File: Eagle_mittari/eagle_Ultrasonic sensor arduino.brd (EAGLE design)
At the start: 69.5 x 55.9 mm, 3 parts

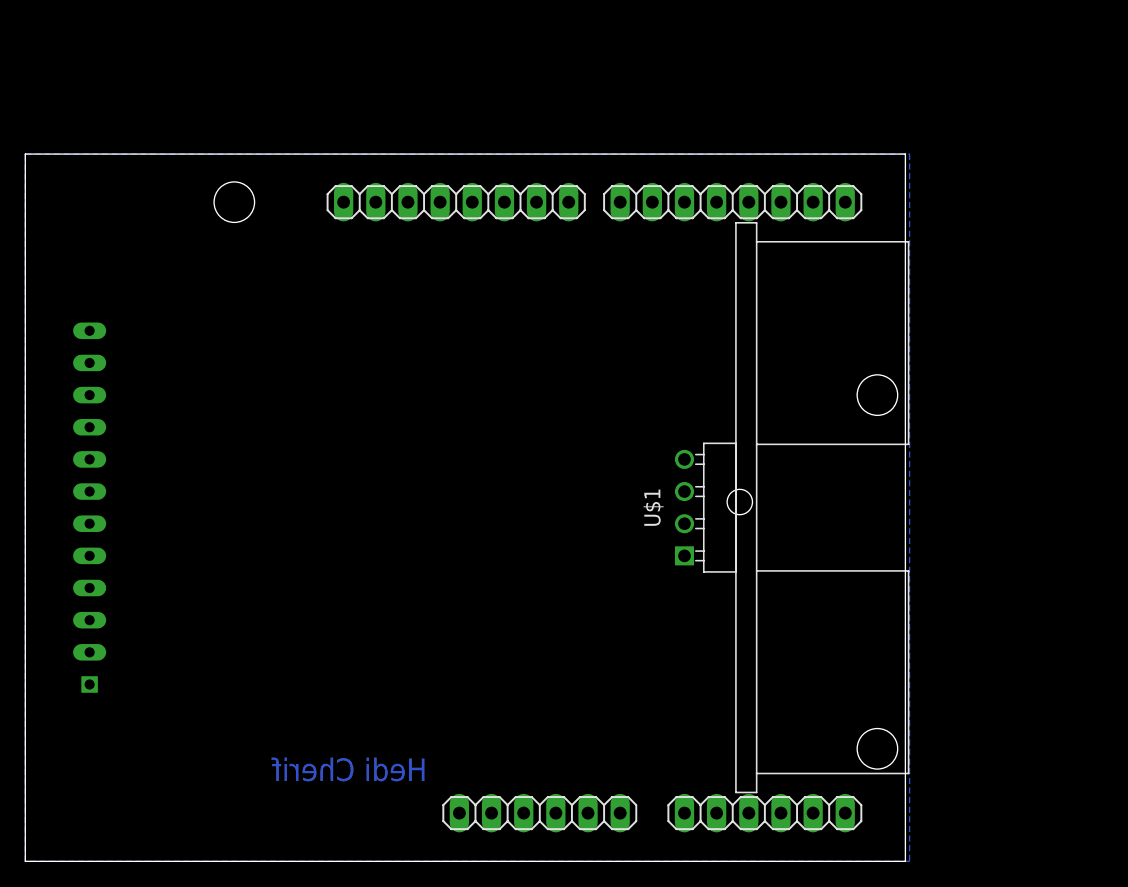
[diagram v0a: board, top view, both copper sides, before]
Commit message: valmistus
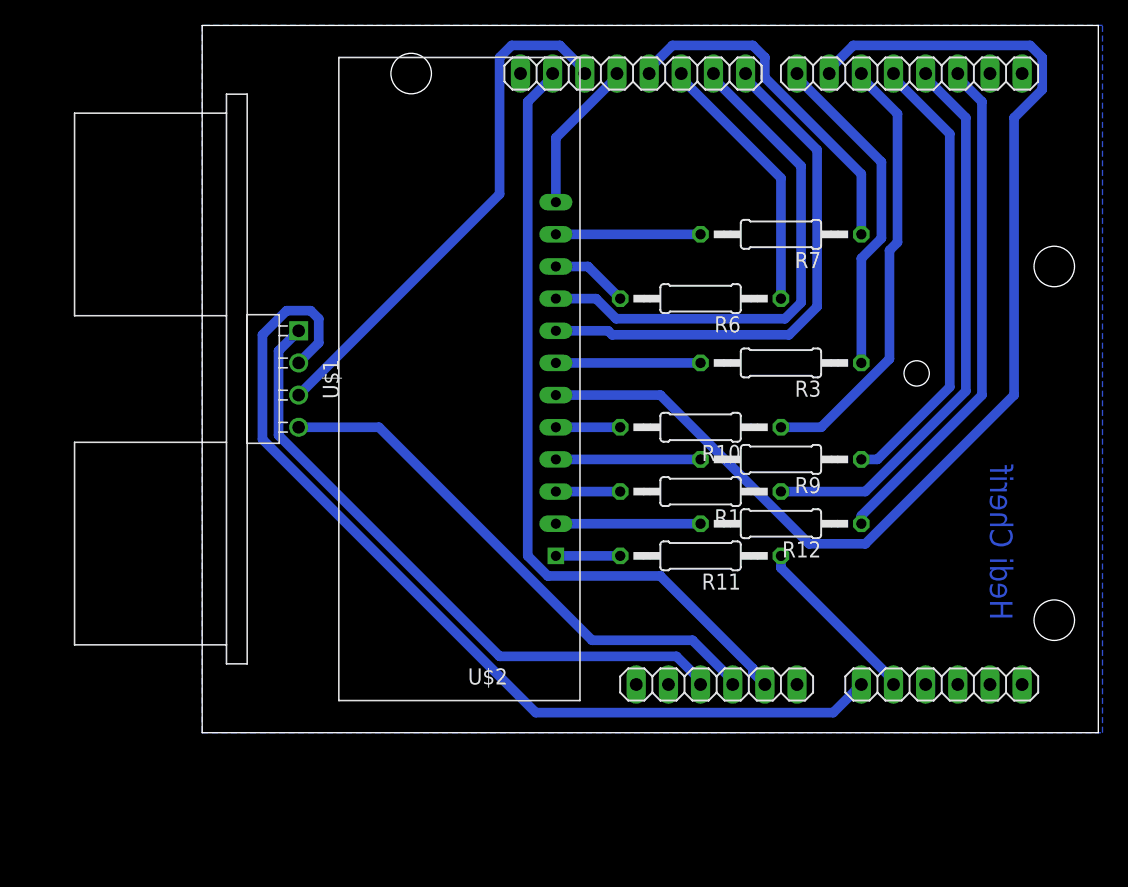
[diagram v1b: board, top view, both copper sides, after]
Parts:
- added R1, R10, R11, R12, R9: 150, rcl:0207/12
- added R3, R6, R7: (no value), rcl:0207/12
- moved U$1 32.1 mm to (20.3, 36.8), turned to 270 degrees
- moved U$2 23.9 mm to (33.0, 36.8), flipped to the top
- moved IC2 17.3 mm to (14.0, 10.2)
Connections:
- removed net N$5 (its old number): IC2.14, U$2.P$1
- new net N$15: IC2.8, R11.1
- new net N$18: IC2.24, R7.1
- new net N$19: IC2.23, R6.1
- new net N$22: IC2.20, R3.1
- new net N$24: IC2.15, R12.1
- new net N$25: IC2.16, R1.1
- new net N$26: IC2.17, R9.1
- new net N$27: IC2.18, R10.1
- new net N$28: R11.2, U$2.P$1
- net N$1: now also R7.2; no longer IC2.24
- net N$2: now also R3.2; no longer IC2.20
- net N$3: now also R9.2; no longer IC2.17
- net N$4: now also R12.2; no longer IC2.15
- net N$6: now also R6.2; no longer IC2.23
- net N$7: now also R10.2; no longer IC2.18
- net N$8: now also R1.2; no longer IC2.16
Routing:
- net N$12: track 0.00 -> 91.8 mm
- net N$5: track 0.00 -> 75.1 mm
- net GND: track 0.00 -> 62.4 mm
- net N$14: track 0.00 -> 50.6 mm
- net N$25: track 0.00 -> 44.3 mm
- net N$13: track 0.00 -> 42.9 mm
- net N$11: track 0.00 -> 42.6 mm
- net N$16: track 0.00 -> 41.8 mm
- net N$10: track 0.00 -> 41.7 mm
- net N$24: track 0.00 -> 40.3 mm
- net N$26: track 0.00 -> 36.0 mm
- net N$27: track 0.00 -> 34.8 mm
- net N$18: track 0.00 -> 28.0 mm
- net N$22: track 0.00 -> 26.3 mm
- net N$19: track 0.00 -> 21.2 mm
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- added copper zone on layer 16, net N$17
- removed copper zone on layer 16, net GND
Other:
- board size 69.5 x 55.9 mm -> 70.8 x 55.9 mm
